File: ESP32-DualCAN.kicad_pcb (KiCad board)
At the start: 2 copper layers, 19.6 x 44.5 mm, 50 parts, among them J1 USB_C_Receptacle_USB2.0_14P, J2 705510040, J3 holes, J4 holes, J5 pads, J6 Aux1, SW1 Rst, SW2 Boot, U1 LV2862Y, U2 ESP32-C6-MINI-1, U3 SN65HVD230, U4 SN65HVD230

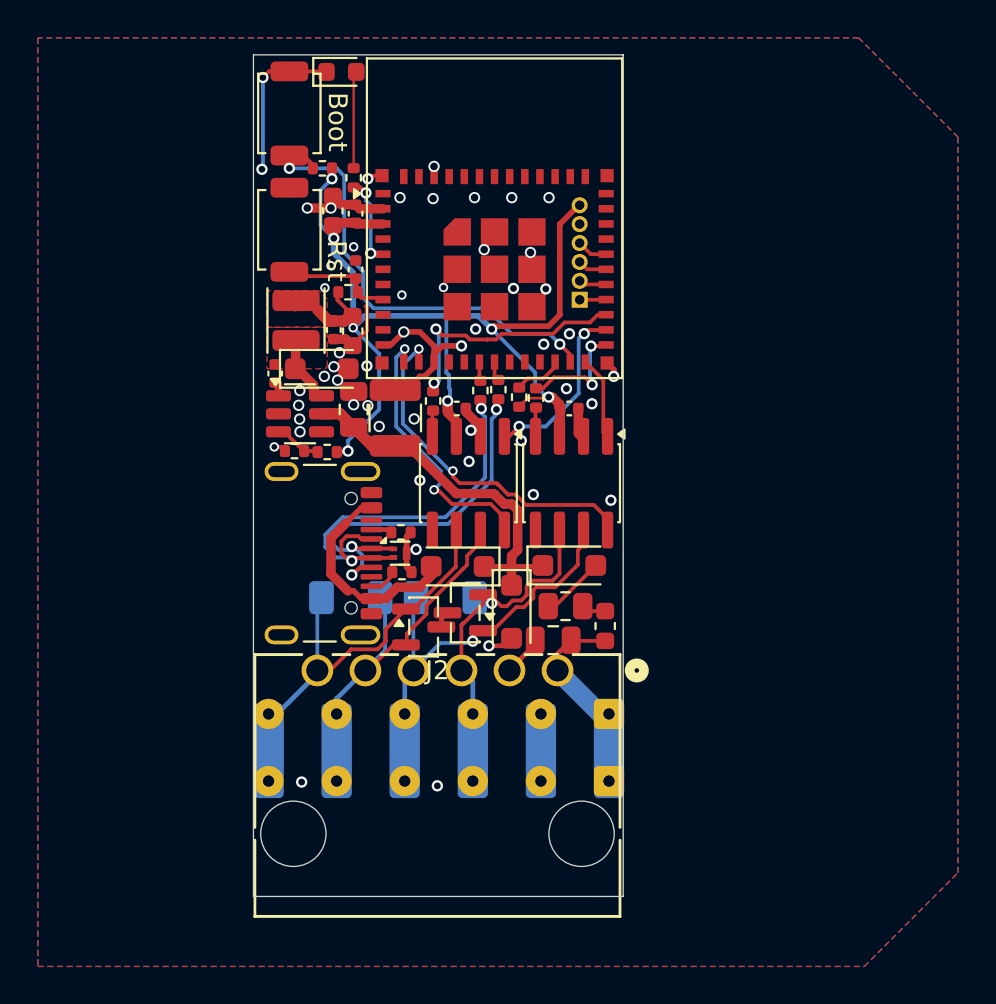
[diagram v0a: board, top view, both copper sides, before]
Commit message: ESP32-C6-Zero main
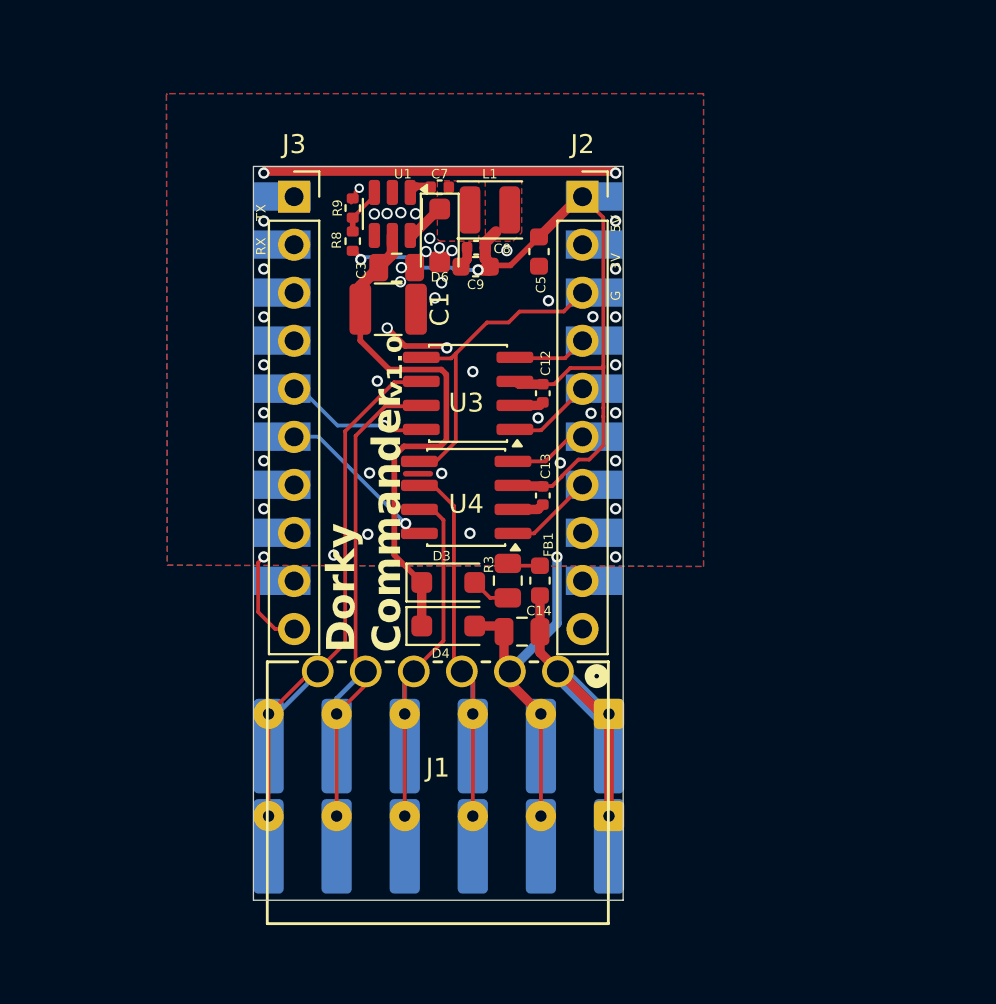
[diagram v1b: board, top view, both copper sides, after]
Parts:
- removed ?: , clipboard:fc211d7d-06df-4809-892a-d774031bd53d
- removed C4, C6: 100n, Capacitor_SMD:C_0402_1005Metric
- removed D1: ESDA5V3L, Package_DFN_QFN:Diodes_DFN1006-3
- removed D2: DSK38, Diode_SMD:D_SOD-123F
- removed D5: Yellow, LED_SMD:LED_0603_1608Metric
- removed D7, D8: H5VNT2B, Package_TO_SOT_SMD:SOT-23
- removed the J1 at (122.1, 99.7)
- removed the J6 at (136.8, 86.3)
- removed R1, R2: 5.11K, Resistor_SMD:R_0402_1005Metric
- removed R10, R11, R7: 470, Resistor_SMD:R_0402_1005Metric
- removed R12, R13: 120Ω, Resistor_SMD:R_1206_3216Metric_Pad1.30x1.75mm_HandSolder
- removed R14, R15: 22, Resistor_SMD:R_0402_1005Metric
- removed R4: 51k, Resistor_SMD:R_0402_1005Metric
- removed R5, R6: 10k, Resistor_SMD:R_0402_1005Metric
- removed REF**: OSHW-Logo2_7.3x6mm_SilkScreen, Symbol:OSHW-Logo2_7.3x6mm_SilkScreen
- removed SW1: Rst, Button_Switch_SMD:SW_SPST_TS-1088-xR020
- removed SW2: Boot, Button_Switch_SMD:SW_SPST_TS-1088-xR020
- added J2: Conn_01x10_Socket, Connector_PinSocket_2.54mm:PinSocket_1x10_P2.54mm_Vertical, F.Cu at (136.9, 80.8)
- added J3: Conn_01x10_Socket, Connector_PinSocket_2.54mm:PinSocket_1x10_P2.54mm_Vertical, F.Cu at (121.7, 80.8)
- added J7: pads, Connector_Wire:SolderWire-0.1sqmm_1x06_P3.6mm_D0.4mm_OD1mm, B.Cu at (138.3, 115.2)
- J1: renamed from J2; value 705510040 -> Molex 70553 6p; footprint lib:CONN_70551-xxxx_06_MOL -> lib:CONN_705530005_06_MOL
- R8: value 51k -> 68k
- R9: value 15k -> 12k
- U2: value ESP32-C6-MINI-1 -> ESP32-C6-Zero; footprint RF_Module:ESP32-C6-MINI-1 -> Waveshare-ESP32:Waveshare-ESP32-C6-Zero; moved to B.Cu
- U3, U4: value SN65HVD230 -> TCAN1044AV
- moved R9 13.2 mm to (124.8, 81.5), turned to -90 degrees
- moved C7 13.1 mm to (129.3, 80.3), turned to 0 degrees
- moved L1 11.8 mm to (132.0, 81.5), turned to 0 degrees
- moved U1 11.6 mm to (126.8, 81.8), turned to -90 degrees
- moved R8 11.2 mm to (124.8, 83.2), turned to -90 degrees
- moved C5 11.1 mm to (134.6, 83.8), turned to -90 degrees
- moved D6 9.41 mm to (129.3, 82.9), turned to -90 degrees
- moved C8 8.69 mm to (131.3, 83.5), turned to 180 degrees
- moved C3 7.84 mm to (127.1, 84.6), turned to 0 degrees
- moved C9 7.34 mm to (131.2, 84.5), turned to 180 degrees
- moved U2 6.55 mm to (129.8, 90.8), turned to 180 degrees
- moved D3 6.46 mm to (129.8, 101.2)
- moved C1 5.76 mm to (126.6, 86.8), turned to 0 degrees
- moved U4 5.62 mm to (130.8, 96.8), turned to 180 degrees
- moved C13 4.81 mm to (134.8, 96.7), turned to -90 degrees
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- renumbered J3 to J4, J4 to J6
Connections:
- C12 pad 1: +3.3V -> +5V
- C13 pad 1: +3.3V -> +5V
- C5 pad 1: +3.3V -> +5V
- C8 pad 1: +3.3V -> +5V
- C9 pad 1: +3.3V -> +5V
- L1 pad 2: +3.3V -> +5V
- R8 pad 2: +3.3V -> +5V
- U2 pad 1: GND -> +5V
- U2 pad 10: unconnected-(U2-IO5-Pad10) -> Net-(J3-Pin_9)
- U2 pad 11: GND -> Net-(J3-Pin_8)
- U2 pad 12: CAN0_RS -> Net-(J3-Pin_7)
- U2 pad 14: GND -> CAN0_RS
- U2 pad 15: unconnected-(U2-IO6-Pad15) -> Net-(J3-Pin_4)
- U2 pad 16: unconnected-(U2-IO7-Pad16) -> Net-(J3-Pin_3)
- U2 pad 4: unconnected-(U2-NC-Pad4) -> CAN0_RXD
- U2 pad 5: Net-(U2-IO2) -> CAN0_TXD
- U2 pad 6: unconnected-(U2-IO3-Pad6) -> CAN1_RXD
- U2 pad 7: unconnected-(U2-NC-Pad7) -> CAN1_TXD
- U2 pad 9: unconnected-(U2-IO4-Pad9) -> Net-(J2-Pin_9)
- U3 pad 3: +3.3V -> +5V
- U3 pad 4: Net-(U3-R) -> CAN0_RXD
- U3 pad 5: unconnected-(U3-Vref-Pad5) -> +3.3V
- U4 pad 3: +3.3V -> +5V
- U4 pad 4: Net-(U4-R) -> CAN1_RXD
- U4 pad 5: unconnected-(U4-Vref-Pad5) -> +3.3V
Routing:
- net +3.3V: track 60.8 -> 17.0 mm, vias 7 -> 0
- net +5V: track 0.00 -> 42.3 mm, vias 0 -> 2
- net Net-(U2-IO9): track 24.9 -> 0.00 mm, vias 2 -> 0
- net USB_D-: track 21.6 -> 0.00 mm, vias 2 -> 0
- net USB_D+: track 21.2 -> 0.00 mm, vias 3 -> 0
- net GND: track 38.3 -> 52.0 mm, vias 52 -> 47
- net CAN0_L: track 22.8 -> 35.0 mm
- net Net-(D2-A): track 11.5 -> 0.00 mm
- net CAN0_H: track 21.3 -> 31.9 mm
- net +BATT: track 10.7 -> 20.4 mm
- net CAN0_RXD: track 13.1 -> 3.97 mm, vias 2 -> 0
- net CAN1_RS: track 18.7 -> 9.67 mm, vias 2 -> 1
- net /BATT_Diode: track 19.8 -> 27.7 mm
- net CAN0_RS: track 14.4 -> 7.65 mm, vias 2 -> 1
- net Net-(J2-Pin_8): track 6.80 -> 0.00 mm
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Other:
- board size 19.6 x 44.5 mm -> 19.6 x 38.8 mm
- board text added: "5V 3V G"
- board text added: "G 3V 5V"
- board text added: "RX TX"
- board text added: "TX RX"
- board text added: "Works with ESP32-C6-Zero in the back or ESP32-C6-SuperMini on the front terminals"
- board text removed: "3.3 G TX0 RX0 TX1 RX1"
